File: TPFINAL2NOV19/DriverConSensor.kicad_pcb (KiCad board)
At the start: 2 copper layers, 77 x 67 mm, 53 parts, among them J1 PULS1, J2 PULS2, J3 MotorT2, J4 MotorT1, J5 VIn+12, J6 Contac12V, J7 GND, K1 Switch de Encendido, K2 FRS10CS10-12V, K3 FRS10CS10-12V, Q1 BC337, Q2 BC337, SW1 SW_DIP_x06, U1 PIC12F675-IP, U2 L78L05_TO92, U3 ACS714T-30A

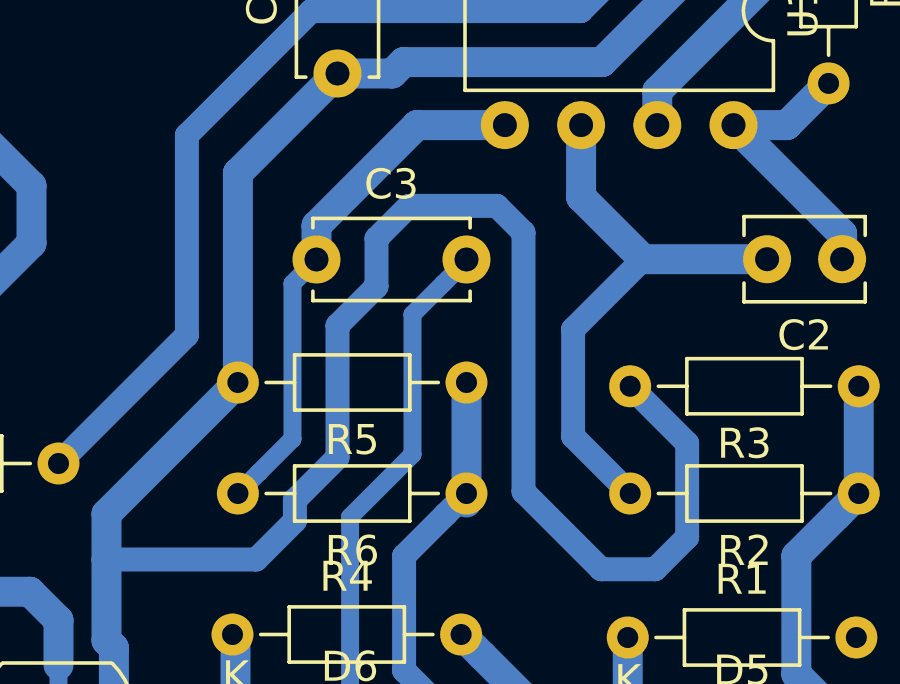
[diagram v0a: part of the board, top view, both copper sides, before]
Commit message: PCB_casi_listo5
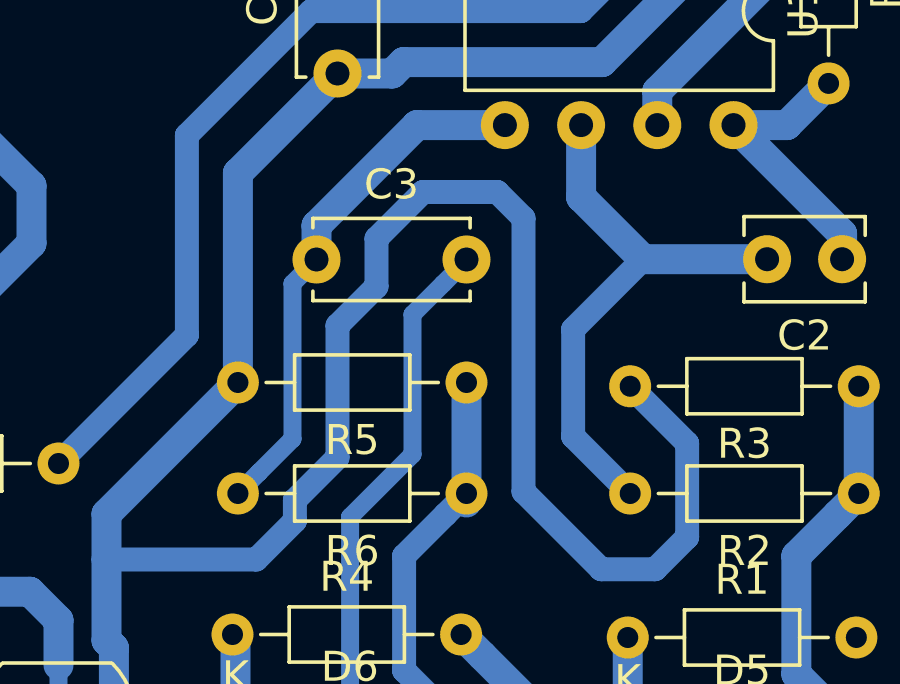
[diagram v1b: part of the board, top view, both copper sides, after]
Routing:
- net +5V: track 213.5 -> 214.2 mm
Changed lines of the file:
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@@
   )
   (setup
-    (last_trace_width 0.6)
+    (last_trace_width 0.8)
     (user_trace_width 0.6)
     (user_trace_width 0.8)
@@
       (effects (font (size 1 1) (thickness 0.15)))
     )
-    (fp_text user %R (at 0 0) (layer F.Fab)
+    (fp_text user GND (at 0 0) (layer F.Fab)
       (effects (font (size 1 1) (thickness 0.15)))
     )
@@
     (fp_line (start -1.5 -1.5) (end -1.5 1.5) (layer F.CrtYd) (width 0.05))
     (fp_line (start -1.5 -1.5) (end 1.5 -1.5) (layer F.CrtYd) (width 0.05))
-    (fp_text user %R (at 0 0) (layer F.Fab)
+    (fp_text user GND (at 0 0) (layer F.Fab)
       (effects (font (size 1 1) (thickness 0.15)))
     )
@@
       (effects (font (size 1 1) (thickness 0.15)))
     )
-    (fp_text user %R (at 1.25 0 90) (layer F.Fab)
+    (fp_text user %R (at 1.25 0 180) (layer F.Fab)
       (effects (font (size 0.76 0.76) (thickness 0.114)))
     )
@@
     (fp_line (start 3.55 1.55) (end 3.55 -1.55) (layer F.CrtYd) (width 0.05))
     (fp_line (start 3.55 -1.55) (end -1.05 -1.55) (layer F.CrtYd) (width 0.05))
-    (fp_text user %R (at 1.25 0 90) (layer F.Fab)
+    (fp_text user %R (at 1.25 0 180) (layer F.Fab)
       (effects (font (size 0.76 0.76) (thickness 0.114)))
     )
@@
       (effects (font (size 1 1) (thickness 0.15)))
     )
-    (fp_text user %R (at 0 0) (layer F.Fab)
+    (fp_text user M1 (at 0 0) (layer F.Fab)
       (effects (font (size 1 1) (thickness 0.15)))
     )
@@
     (fp_line (start -2.75 -2.75) (end -2.75 2.75) (layer F.CrtYd) (width 0.05))
     (fp_line (start -2.75 -2.75) (end 2.75 -2.75) (layer F.CrtYd) (width 0.05))
-    (fp_text user %R (at 0 0) (layer F.Fab)
+    (fp_text user M2 (at 0 0) (layer F.Fab)
       (effects (font (size 1 1) (thickness 0.15)))
     )
@@
       (effects (font (size 1 1) (thickness 0.15)))
     )
-    (fp_text user %R (at 0 0) (layer F.Fab)
+    (fp_text user 12v (at 0 0) (layer F.Fab)
       (effects (font (size 1 1) (thickness 0.15)))
     )
@@
       (effects (font (size 0.8 0.8) (thickness 0.1)))
     )
-    (fp_text user %R (at 0 0) (layer F.Fab)
-      (effects (font (size 1 1) (thickness 0.15)))
+    (fp_text user Cont12V (at 0 0) (layer F.Fab)
+      (effects (font (size 0.8 0.8) (thickness 0.1)))
     )
     (fp_line (start -2.25 -2.25) (end 2.25 -2.25) (layer F.CrtYd) (width 0.05))
@@
     (fp_line (start -2.75 -2.75) (end -2.75 2.75) (layer F.CrtYd) (width 0.05))
     (fp_line (start -2.75 -2.75) (end 2.75 -2.75) (layer F.CrtYd) (width 0.05))
-    (fp_text user %R (at 0 0) (layer F.Fab)
+    (fp_text user GND (at 0 0) (layer F.Fab)
       (effects (font (size 1 1) (thickness 0.15)))
     )
@@
   (segment (start 167.08 103.3) (end 162.70001 107.67999) (width 1) (layer B.Cu) (net 2))
   (segment (start 162.70001 107.67999) (end 162.70001 109.20001) (width 1) (layer B.Cu) (net 2))
-  (segment (start 176.600001 98.300001) (end 175.712699 97.412699) (width 0.8) (layer B.Cu) (net 2))
-  (segment (start 182.055001 105.325001) (end 182.055001 108.456999) (width 0.8) (layer B.Cu) (net 2))
-  (segment (start 182.055001 108.456999) (end 180.987001 109.524999) (width 0.8) (layer B.Cu) (net 2))
-  (segment (start 180.987001 109.524999) (end 179.187753 109.524999) (width 0.8) (layer B.Cu) (net 2))
-  (segment (start 180.155 103.425) (end 182.055001 105.325001) (width 0.8) (layer B.Cu) (net 2))
-  (segment (start 179.187753 109.524999) (end 176.600001 106.937247) (width 0.8) (layer B.Cu) (net 2))
-  (segment (start 176.600001 106.937247) (end 176.600001 98.300001) (width 0.8) (layer B.Cu) (net 2))
-  (segment (start 167.691992 109.20001) (end 162.70001 109.20001) (width 0.8) (layer B.Cu) (net 2))
-  (segment (start 168.980001 107.912001) (end 167.691992 109.20001) (width 0.8) (layer B.Cu) (net 2))
-  (segment (start 168.980001 107.221333) (end 168.980001 107.912001) (width 0.8) (layer B.Cu) (net 2))
-  (segment (start 170.40001 105.801324) (end 168.980001 107.221333) (width 0.8) (layer B.Cu) (net 2))
-  (segment (start 170.400011 101.399989) (end 170.40001 105.801324) (width 0.8) (layer B.Cu) (net 2))
-  (segment (start 171.700001 100.099999) (end 170.400011 101.399989) (width 0.8) (layer B.Cu) (net 2))
-  (segment (start 171.700001 98.499999) (end 171.700001 100.099999) (width 0.8) (layer B.Cu) (net 2))
-  (segment (start 172.787301 97.412699) (end 171.700001 98.499999) (width 0.8) (layer B.Cu) (net 2))
-  (segment (start 175.712699 97.412699) (end 172.787301 97.412699) (width 0.8) (layer B.Cu) (net 2))
   (segment (start 160.300001 120.000001) (end 158.425001 120.000001) (width 1) (layer B.Cu) (net 2))
   (segment (start 161.1 120.8) (end 160.300001 120.000001) (width 1) (layer B.Cu) (net 2))
@@
   (segment (start 127.53994 97.745) (end 128.45001 98.65507) (width 0.6) (layer B.Cu) (net 2))
   (segment (start 126.35 97.745) (end 127.53994 97.745) (width 0.6) (layer B.Cu) (net 2))
+  (segment (start 168.980001 107.221333) (end 168.980001 107.912001) (width 0.8) (layer B.Cu) (net 2))
+  (segment (start 170.40001 105.801324) (end 168.980001 107.221333) (width 0.8) (layer B.Cu) (net 2))
+  (segment (start 170.400011 101.399989) (end 170.40001 105.801324) (width 0.8) (layer B.Cu) (net 2))
+  (segment (start 171.700001 100.099999) (end 170.400011 101.399989) (width 0.8) (layer B.Cu) (net 2))
+  (segment (start 173.25 96.95) (end 171.700001 98.499999) (width 0.8) (layer B.Cu) (net 2))
+  (segment (start 182.055001 105.325001) (end 182.055001 108.456999) (width 0.8) (layer B.Cu) (net 2))
+  (segment (start 168.980001 107.912001) (end 167.691992 109.20001) (width 0.8) (layer B.Cu) (net 2))
+  (segment (start 180.155 103.425) (end 182.055001 105.325001) (width 0.8) (layer B.Cu) (net 2))
+  (segment (start 167.691992 109.20001) (end 162.70001 109.20001) (width 0.8) (layer B.Cu) (net 2))
+  (segment (start 176.600001 97.825001) (end 175.725 96.95) (width 0.8) (layer B.Cu) (net 2))
+  (segment (start 180.987001 109.524999) (end 179.187753 109.524999) (width 0.8) (layer B.Cu) (net 2))
+  (segment (start 171.700001 98.499999) (end 171.700001 100.099999) (width 0.8) (layer B.Cu) (net 2))
+  (segment (start 179.187753 109.524999) (end 176.600001 106.937247) (width 0.8) (layer B.Cu) (net 2))
+  (segment (start 175.725 96.95) (end 173.25 96.95) (width 0.8) (layer B.Cu) (net 2))
+  (segment (start 182.055001 108.456999) (end 180.987001 109.524999) (width 0.8) (layer B.Cu) (net 2))
+  (segment (start 176.600001 106.937247) (end 176.600001 97.825001) (width 0.8) (layer B.Cu) (net 2))
   (segment (start 178.52 97.12) (end 178.52 94.72) (width 1) (layer B.Cu) (net 3) (status 20))
   (segment (start 180.59 99.19) (end 178.52 97.12) (width 1) (layer B.Cu) (net 3))
